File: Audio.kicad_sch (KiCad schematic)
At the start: 8 parts, among them T1 SM-LP-5001E, T2 SM-LP-5001E

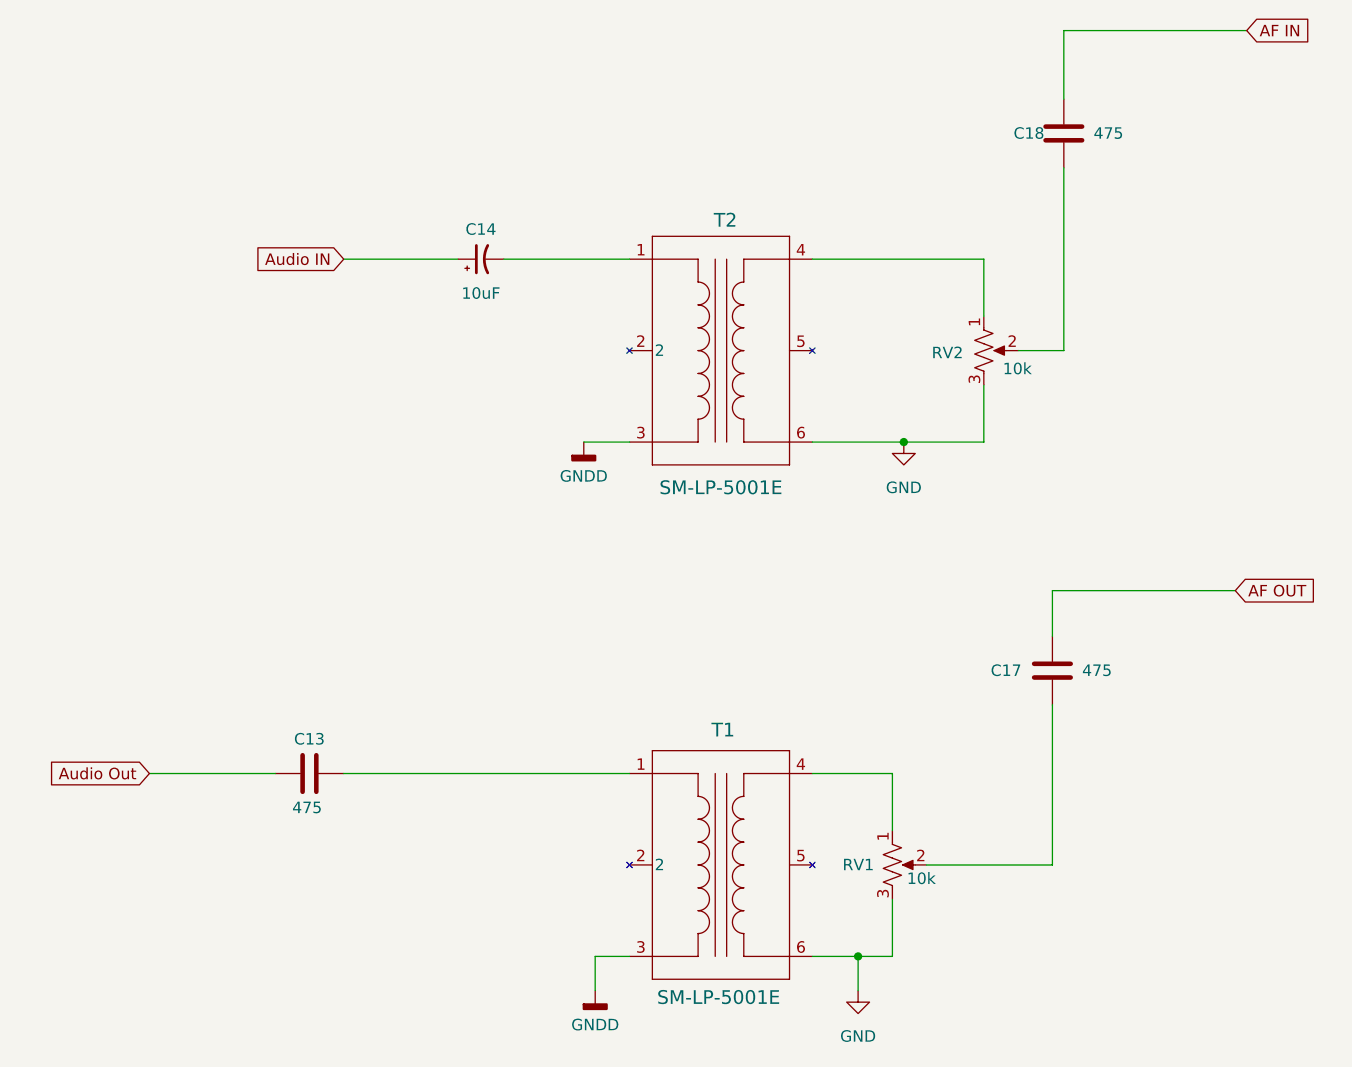
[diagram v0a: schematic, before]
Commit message: kiCAD 9.0
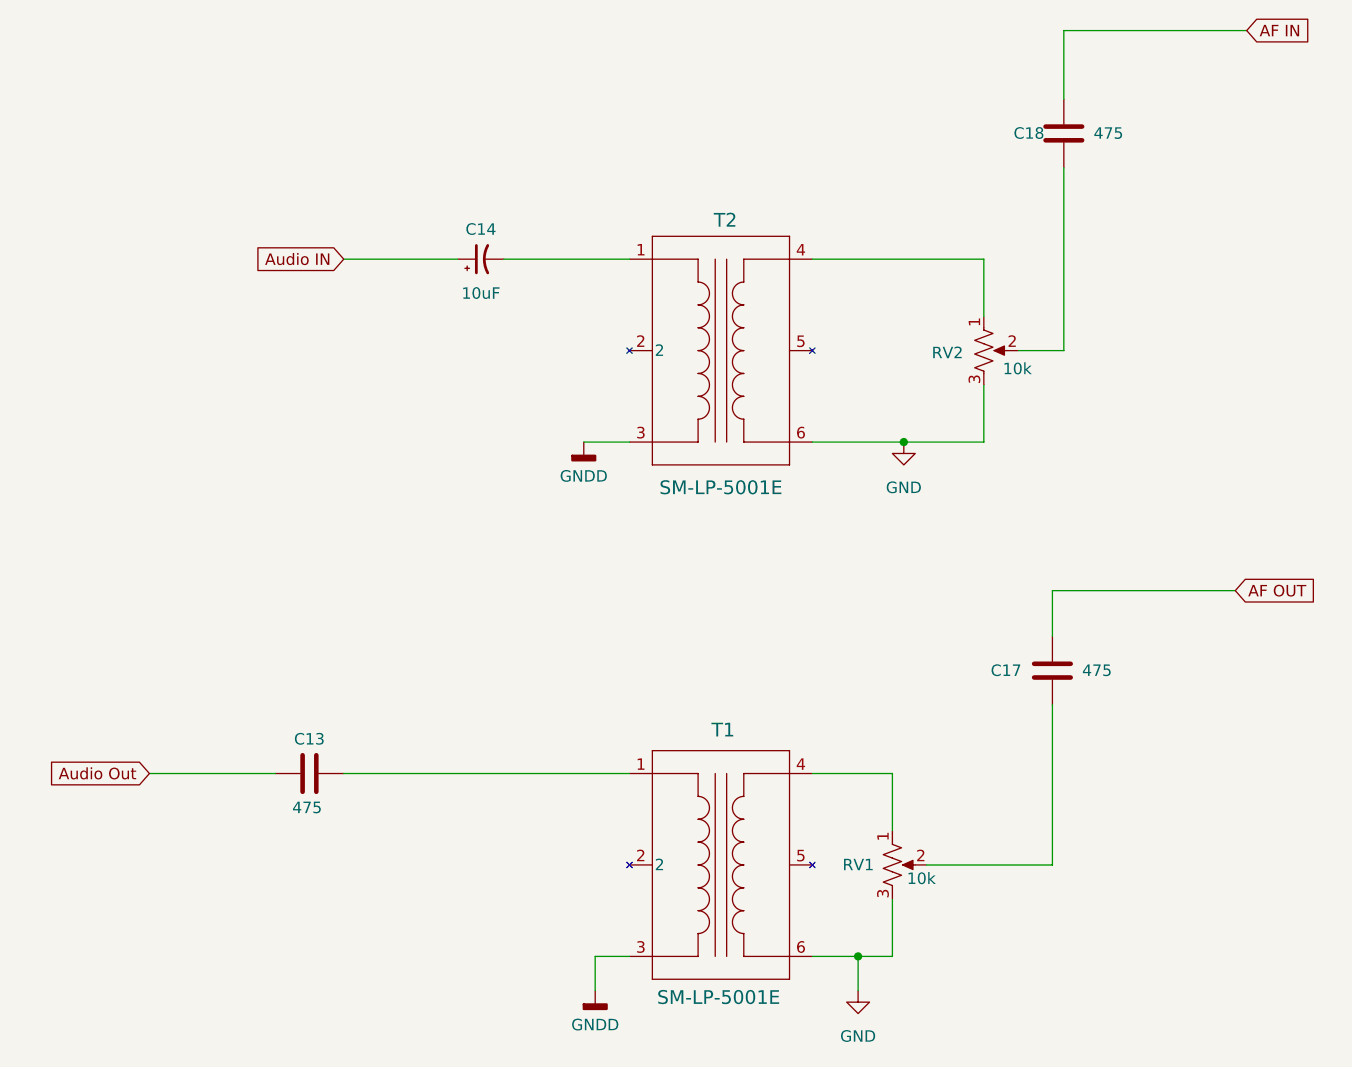
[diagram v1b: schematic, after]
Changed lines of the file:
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@@
 (kicad_sch
-	(version 20231120)
+	(version 20250114)
 	(generator "eeschema")
-	(generator_version "8.0")
+	(generator_version "9.0")
 	(paper "USLetter")
 	(title_block
